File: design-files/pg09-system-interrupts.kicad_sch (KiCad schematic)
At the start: 16 parts, among them U401 W65C21, U402 GAL22V10, U403 GAL22V10, U404 GAL22V10, U405 74AHC374, U406 74AHC374, U407 74AHC138

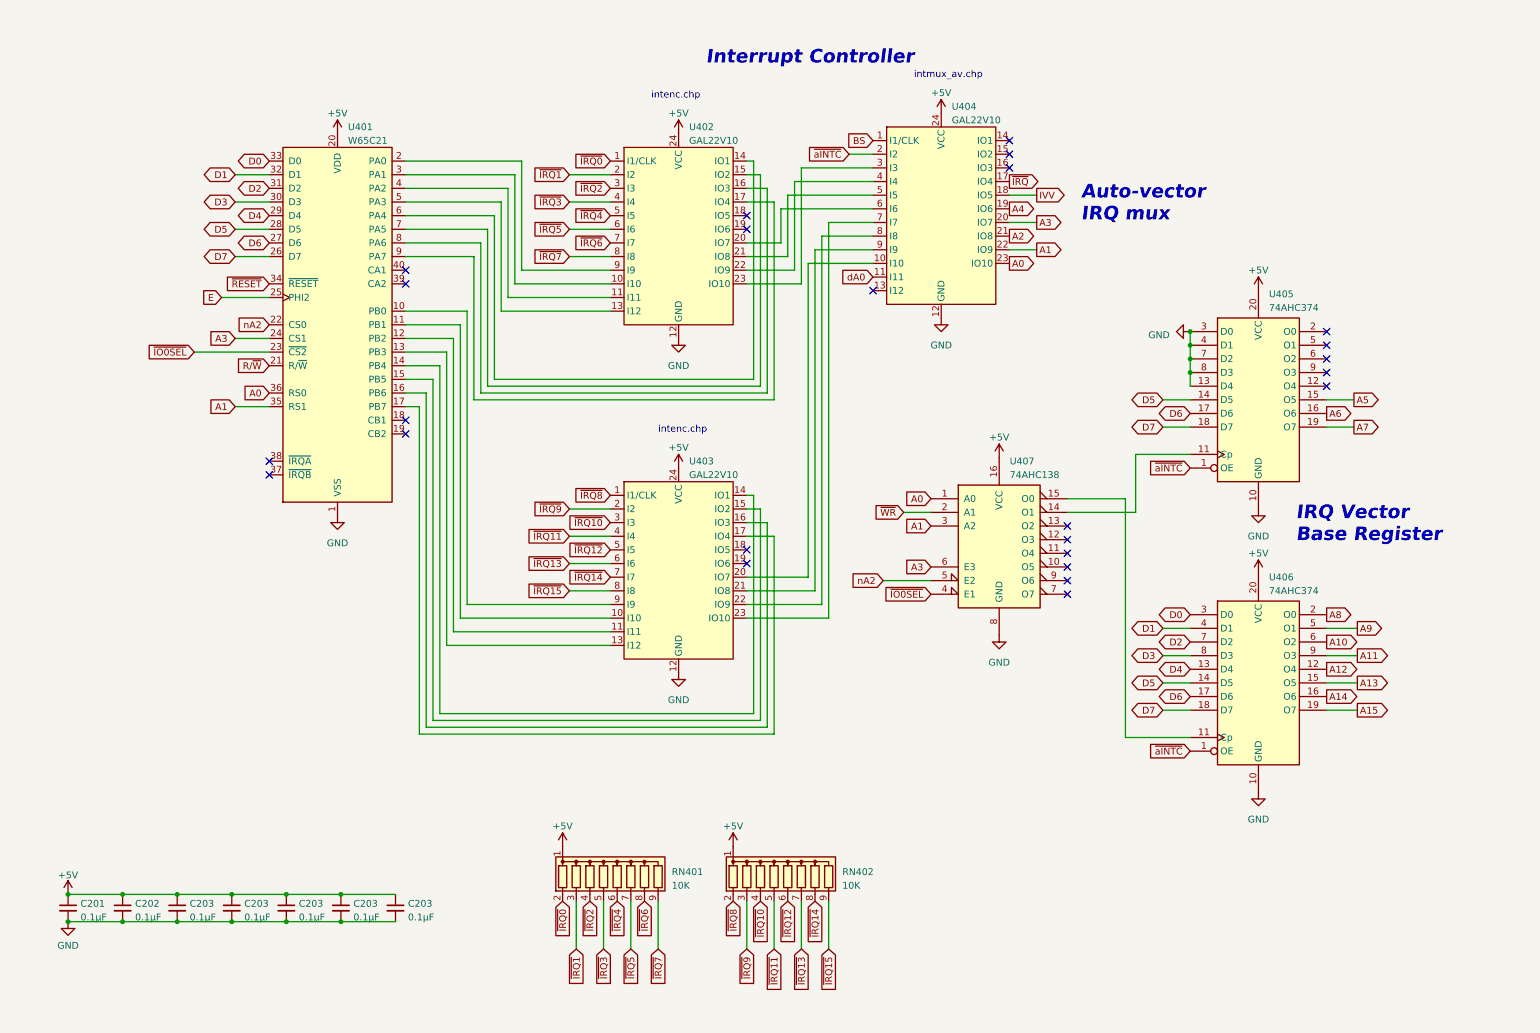
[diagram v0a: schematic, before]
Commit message: Re-work the interrupt controller to use discrete 74xx chips for mixing the enable signals and priority-encoding.
I made a major blunder in the INTENC GAL, and when I went to correct
it, it became clear that putting enable-mixing + priority encoding into
a single 22V10 wasn't going to fit.  At that point, the GAL was going
to be used either for priority encoding OR enable-mixing, and it just
didn't seem worth it.  So, INTENC goes away and is replaced by 74HC04s,
74HC00s, and 74HC148s.  The chip count kind of exploded here with 16
IRQs, but it fits on the board OK and the propagation delay for IRQ
signals doens't matter all that much.

Pay attention do how the 74HC148 is connected and look at the truth table
for that part carefully!
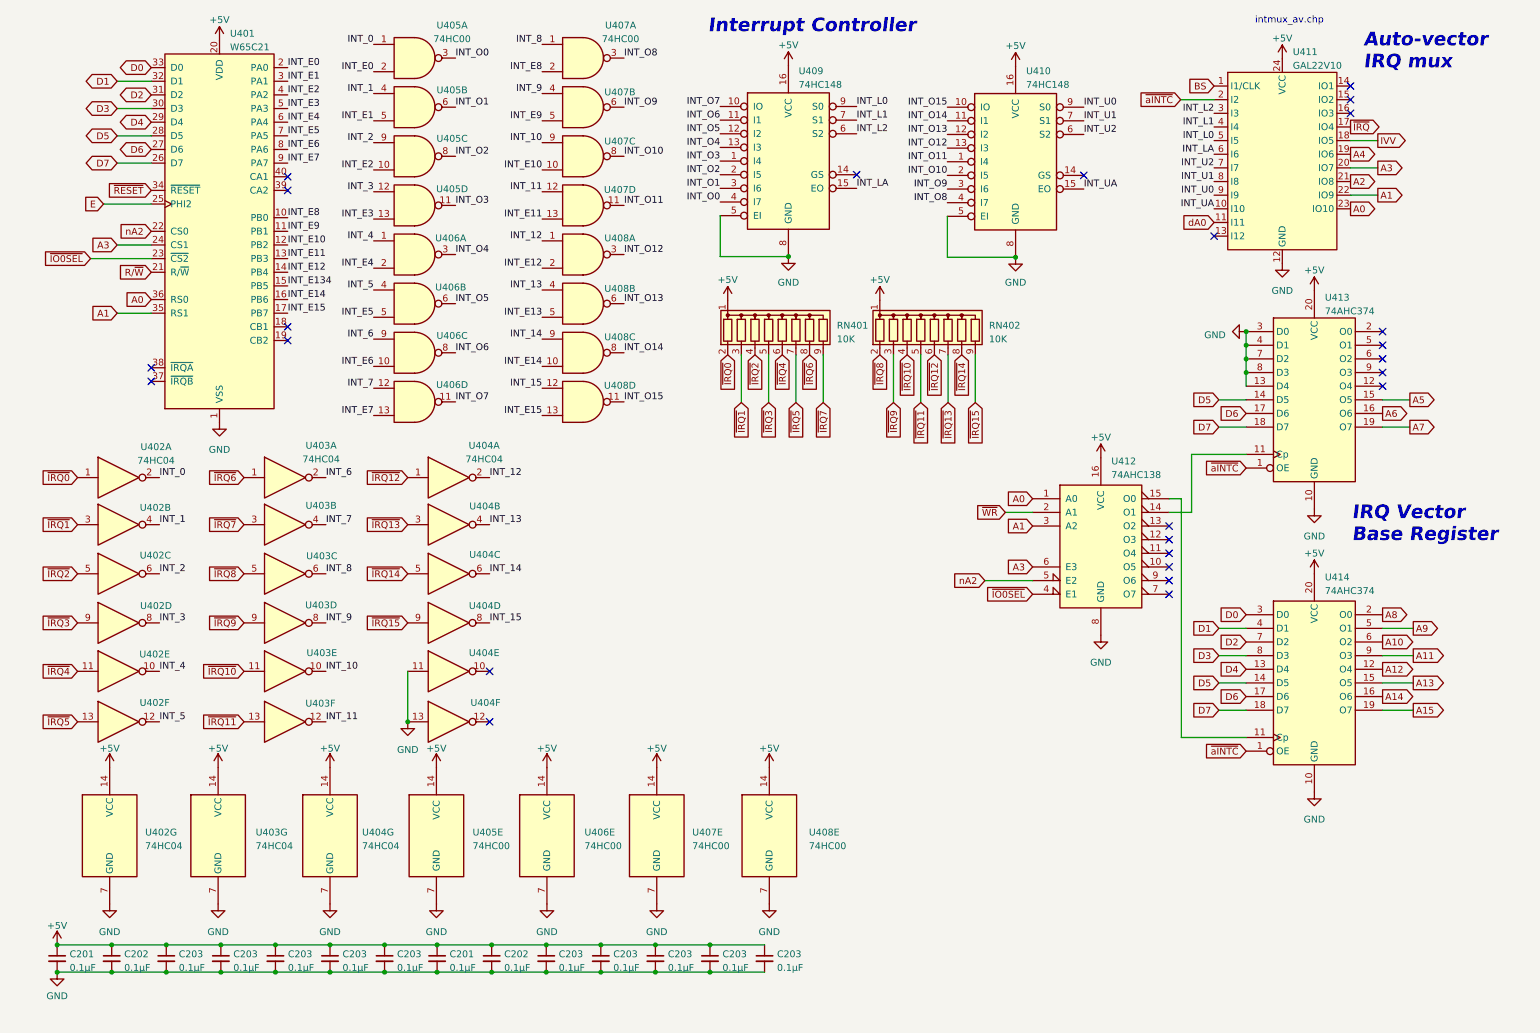
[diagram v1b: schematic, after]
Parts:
- removed U402, U403: GAL22V10, Package_DIP:DIP-24_W7.62mm_Socket, symbol jrt-ICs:GAL22V10
- added C201, C202, C203 (x5): 0.1µF, Capacitor_THT:C_Disc_D3.8mm_W2.6mm_P2.50mm, symbol Device:C_Small
- added U402, U403, U404: 74HC04, Package_DIP:DIP-14_W7.62mm_Socket, symbol 74xx:74HC04
- added U405, U406, U407, U408: 74HC00, Package_DIP:DIP-14_W7.62mm_Socket, symbol 74xx:74HC00
- added U409, U410: 74HC148, Package_DIP:DIP-16_W7.62mm_Socket, symbol 74xx:74LS148
- renumbered U404 to U411, U407 to U412, U405 to U413, U406 to U414
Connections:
- net +5V: now also C201.1, C202.1, C203.1, C203.1, C203.1, C203.1, C203.1, U402.14 (VCC), U403.14 (VCC), U404.14 (VCC), U405.14 (VCC), U406.14 (VCC), U407.14 (VCC), U408.14 (VCC), U409.16 (VCC), U410.16 (VCC)
- net GND: now also C201.2, C202.2, C203.2, C203.2, C203.2, C203.2, C203.2, U402.7 (GND), U403.7 (GND), U404.11, U404.13, U404.7 (GND), U405.7 (GND), U406.7 (GND), U407.7 (GND), U408.7 (GND), U409.5 (EI), U409.8 (GND), U410.5 (EI), U410.8 (GND)
- net ~{IRQ0}: now also U402.1
- net ~{IRQ10}: now also U403.11
- net ~{IRQ11}: now also U403.13
- net ~{IRQ12}: now also U404.1
- net ~{IRQ13}: now also U404.3
- net ~{IRQ14}: now also U404.5
- net ~{IRQ15}: now also U404.9
- net ~{IRQ1}: now also U402.3
- net ~{IRQ2}: now also U402.5
- net ~{IRQ3}: now also U402.9
- net ~{IRQ4}: now also U402.11
- net ~{IRQ5}: now also U402.13
- net ~{IRQ6}: now also U403.1
- net ~{IRQ7}: now also U403.3
- net ~{IRQ8}: now also U403.5
- net ~{IRQ9}: now also U403.9
- net INT_E8: now reaches U401.10 (PB0)
- net INT_E8: now also U407.2
- net INT_E9: now reaches U401.11 (PB1)
- net INT_E9: now also U407.5
- net INT_E10: now reaches U401.12 (PB2)
- net INT_E10: now also U407.10
- net INT_E11: now reaches U401.13 (PB3)
- net INT_E11: now also U407.13
- net INT_E12: now reaches U401.14 (PB4)
- net INT_E12: now also U408.2
- net INT_E134: now reaches U401.15 (PB5)
- net INT_E14: now reaches U401.16 (PB6)
- net INT_E14: now also U408.10
- net INT_E15: now reaches U401.17 (PB7)
- net INT_E15: now also U408.13
- net INT_E0: now reaches U401.2 (PA0)
- net INT_E0: now also U405.2
- net INT_E1: now reaches U401.3 (PA1)
- net INT_E1: now also U405.5
- net INT_E2: now reaches U401.4 (PA2)
- net INT_E2: now also U405.10
- net INT_E3: now reaches U401.5 (PA3)
- net INT_E3: now also U405.13
- net INT_E4: now reaches U401.6 (PA4)
- net INT_E4: now also U406.2
- net INT_E5: now reaches U401.7 (PA5)
- net INT_E5: now also U406.5
- net INT_E6: now reaches U401.8 (PA6)
- net INT_E6: now also U406.10
- net INT_E7: now reaches U401.9 (PA7)
- net INT_E7: now also U406.13
- net INT_UA: now reaches U411.10 (I10)
- net INT_UA: now also U410.15 (EO)
- net INT_L2: now reaches U411.3 (I3)
- net INT_L2: now also U409.6 (S2)
- net INT_L1: now reaches U411.4 (I4)
- net INT_L1: now also U409.7 (S1)
- net INT_L0: now reaches U411.5 (I5)
- net INT_L0: now also U409.9 (S0)
- net INT_LA: now reaches U411.6 (I6)
- net INT_LA: now also U409.15 (EO)
- net INT_U2: now reaches U411.7 (I7)
- net INT_U2: now also U410.6 (S2)
- net INT_U1: now reaches U411.8 (I8)
- net INT_U1: now also U410.7 (S1)
- net INT_U0: now reaches U411.9 (I9)
- net INT_U0: now also U410.9 (S0)
- new net INT_0: U402.2, U405.1
- new net INT_1: U402.4, U405.4
- new net INT_10: U403.10, U407.9
- new net INT_11: U403.12, U407.12
- new net INT_12: U404.2, U408.1
- new net INT_13: U404.4, U408.4
- new net INT_14: U404.6, U408.9
- new net INT_15: U404.8, U408.12
- new net INT_2: U402.6, U405.9
- new net INT_3: U402.8, U405.12
- new net INT_4: U402.10, U406.1
- new net INT_5: U402.12, U406.4
- new net INT_6: U403.2, U406.9
- new net INT_7: U403.4, U406.12
- new net INT_8: U403.6, U407.1
- new net INT_9: U403.8, U407.4
- new net INT_E13: U408.5
- new net INT_O0: U405.3, U409.4 (I7)
- new net INT_O1: U405.6, U409.3 (I6)
- new net INT_O10: U407.8, U410.2 (I5)
- new net INT_O11: U407.11, U410.1 (I4)
- new net INT_O12: U408.3, U410.13 (I3)
- new net INT_O13: U408.6, U410.12 (I2)
- new net INT_O14: U408.8, U410.11 (I1)
- new net INT_O15: U408.11, U410.10 (IO)
- new net INT_O2: U405.8, U409.2 (I5)
- new net INT_O3: U405.11, U409.1 (I4)
- new net INT_O4: U406.3, U409.13 (I3)
- new net INT_O5: U406.6, U409.12 (I2)
- new net INT_O6: U406.8, U409.11 (I1)
- new net INT_O7: U406.11, U409.10 (IO)
- new net INT_O8: U407.3, U410.4 (I7)
- new net INT_O9: U407.6, U410.3 (I6)
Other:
- note removed: "intenc.chp"
- moved on the sheet: C201, C202, C203, RN401, RN402, U401, U411, U412, U413, U414
